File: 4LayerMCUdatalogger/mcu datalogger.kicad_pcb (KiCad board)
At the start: 4 copper layers, 50.3 x 32 mm, 29 parts, among them J1 Conn_01x04_Pin, J2 Conn_01x09_Pin, J3 Conn_01x04_Pin, J4 Conn_02x03_Odd_Even, U1 24LC1025, U2 DS1337S_, U3 24LC1025, U4 ATMEGA328P-AU, Y1 32.768 KHz, Y2 16MHz

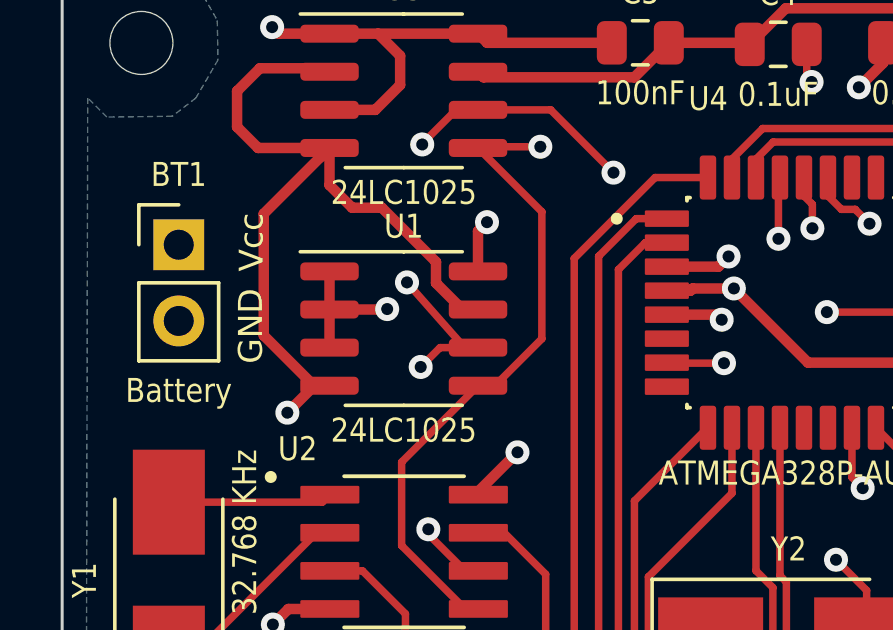
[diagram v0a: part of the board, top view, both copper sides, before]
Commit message: Small modifications.
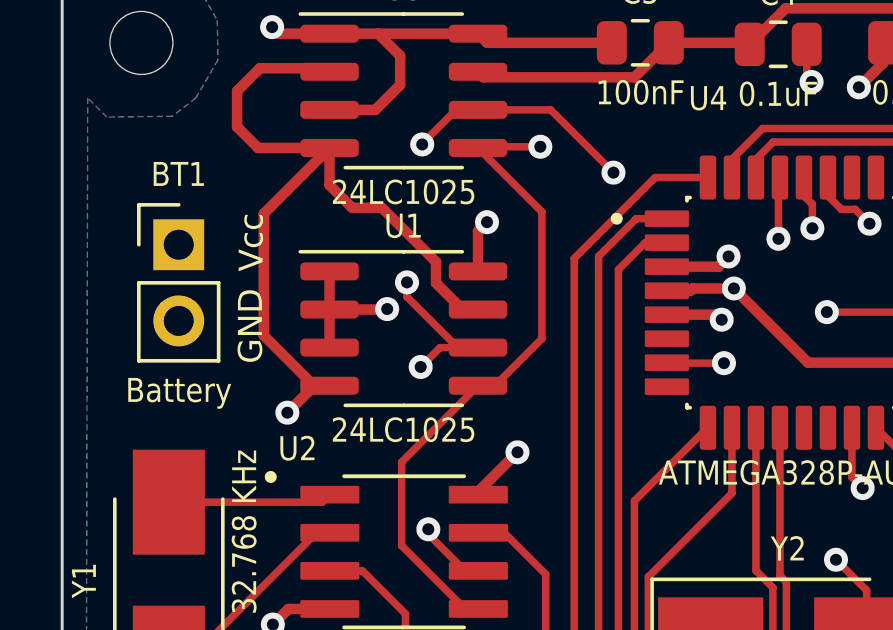
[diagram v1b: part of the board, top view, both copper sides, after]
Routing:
- net /SCL: track 75.8 -> 75.2 mm
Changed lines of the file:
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@@
       (drillshape 0)
       (scaleselection 1)
-      (outputdirectory "mcu datalogger gerbers/")
+      (outputdirectory "4layer_MCU_Datalogger_gerbers/")
     )
   )
@@
   (segment (start 145.764 85.7615) (end 145.764 76.2365) (width 0.25) (layer "In2.Cu") (net 8))
   (segment (start 129.2233 74.7072) (end 129.2233 72.9038) (width 0.25) (layer "In2.Cu") (net 8))
-  (segment (start 115.725738 78.8372) (end 116.1732 78.8372) (width 0.25) (layer "F.Cu") (net 9))
   (segment (start 114.9079 78.8372) (end 114.2627 79.4824) (width 0.25) (layer "F.Cu") (net 9))
   (segment (start 114.5167 85.057126) (end 115.738974 86.2794) (width 0.25) (layer "F.Cu") (net 9))
@@
   (segment (start 134.8875 72.4212) (end 134.8875 72.2688) (width 0.25) (layer "F.Cu") (net 9))
   (segment (start 136.9149 72.5298) (end 135.1485 72.5298) (width 0.25) (layer "F.Cu") (net 9))
+  (segment (start 113.8055 77.1456) (end 115.4971 78.8372) (width 0.25) (layer "F.Cu") (net 9))
+  (segment (start 115.4971 78.8372) (end 115.725738 78.8372) (width 0.25) (layer "F.Cu") (net 9))
   (segment (start 115.4413 70.9124) (end 114.3135 72.0402) (width 0.25) (layer "F.Cu") (net 9))
   (segment (start 127.038 73.1686) (end 127.038 73.780227) (width 0.25) (layer "F.Cu") (net 9))
   (segment (start 120.6889 73.0054) (end 118.5959 70.9124) (width 0.25) (layer "F.Cu") (net 9))
-  (segment (start 113.8055 76.663) (end 115.725738 78.8372) (width 0.25) (layer "F.Cu") (net 9))
   (segment (start 137.9899 73.6048) (end 136.9149 72.5298) (width 0.25) (layer "F.Cu") (net 9))
   (segment (start 135.0399 72.4212) (end 134.8875 72.4212) (width 0.25) (layer "F.Cu") (net 9))
+  (segment (start 113.8055 76.663) (end 113.8055 77.1456) (width 0.25) (layer "F.Cu") (net 9))
   (segment (start 134.8875 72.2688) (end 134.9129 72.2942) (width 0.25) (layer "F.Cu") (net 9))
   (segment (start 146.6027 90.0684) (end 149.3266 90.0684) (width 0.25) (layer "F.Cu") (net 9))
@@
   (segment (start 113.8055 76.663) (end 113.8055 72.5736) (width 0.25) (layer "In1.Cu") (net 9))
   (segment (start 129.7567 72.4212) (end 134.8875 72.4212) (width 0.25) (layer "In1.Cu") (net 9))
-  (segment (start 114.5167 84.8926) (end 114.2627 84.7148) (width 0.25) (layer "In1.Cu") (net 9))
   (segment (start 127.3183 74.8596) (end 129.7567 72.4212) (width 0.25) (layer "In1.Cu") (net 9))
   (segment (start 127.3183 74.8596) (end 126.9431 74.4844) (width 0.25) (layer "In2.Cu") (net 9))
